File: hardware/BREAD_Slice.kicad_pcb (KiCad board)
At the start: 2 copper layers, 70 x 100 mm, 18 parts, among them J1 Conn_01x10_Female, J2 Screw_Terminal_01x02, J3 Screw_Terminal_01x02, U1 AP63205

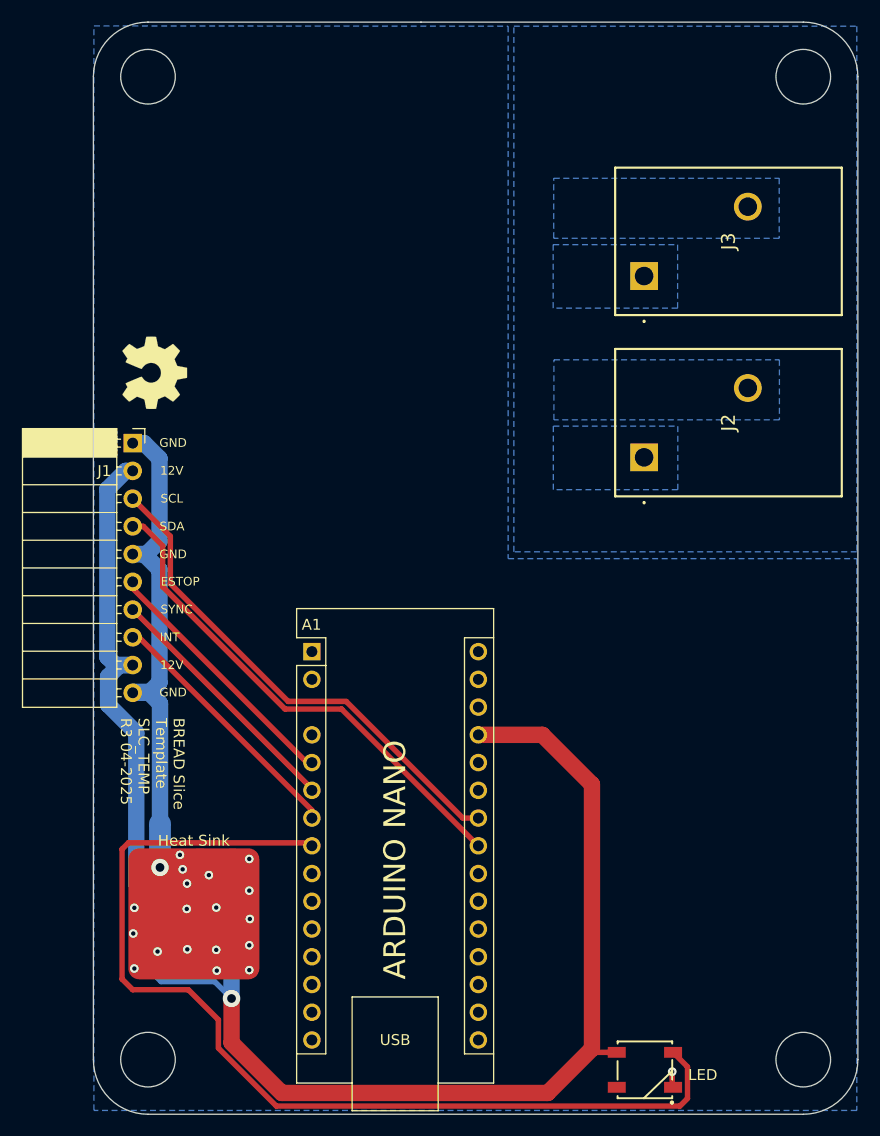
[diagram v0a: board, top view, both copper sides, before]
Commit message: completed board
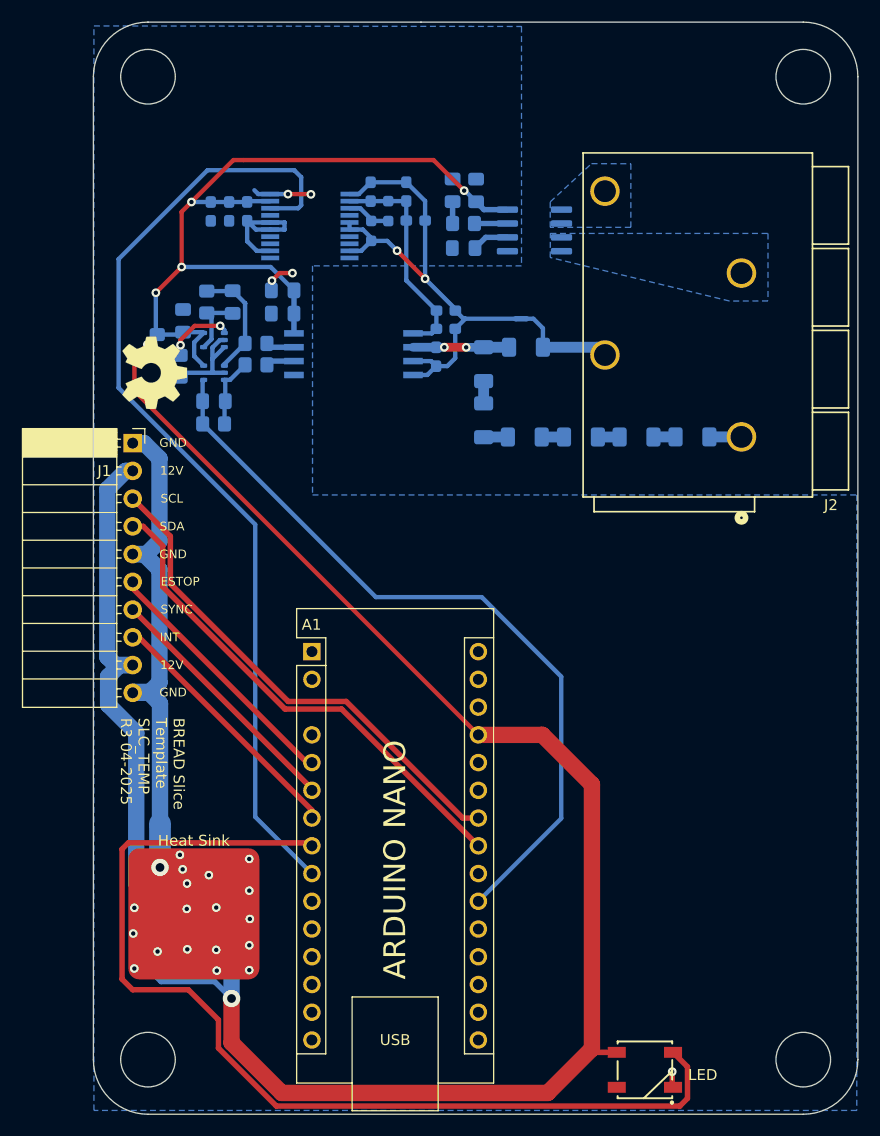
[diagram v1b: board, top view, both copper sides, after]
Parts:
- removed J3: Screw_Terminal_01x02, CRx:Pheonix Conn Term TDPT 4 2-SP-6,35-ZB
- added C10: 100n, Capacitor_SMD:C_0603_1608Metric_Pad1.08x0.95mm_HandSolder, B.Cu at (154.9, 67.9)
- added C11: 0.1u, Capacitor_SMD:C_0603_1608Metric_Pad1.08x0.95mm_HandSolder, B.Cu at (152.1, 58.0)
- added C12: 100p, Capacitor_SMD:C_0603_1608Metric_Pad1.08x0.95mm_HandSolder, B.Cu at (154.0, 70.4)
- added C13: 10n, Capacitor_SMD:C_0603_1608Metric_Pad1.08x0.95mm_HandSolder, B.Cu at (148.0, 55.3)
- added C14: 10n, Capacitor_SMD:C_0603_1608Metric_Pad1.08x0.95mm_HandSolder, B.Cu at (136.7, 57.1)
- added C15: 0.1u, Capacitor_SMD:C_0603_1608Metric_Pad1.08x0.95mm_HandSolder, B.Cu at (135.0, 57.1)
- added C16: 330p, Capacitor_SMD:C_0805_2012Metric_Pad1.18x1.45mm_HandSolder, B.Cu at (135.3, 65.4)
- added C17: 10u, Capacitor_SMD:C_0603_1608Metric_Pad1.08x0.95mm_HandSolder, B.Cu at (133.3, 57.1)
- added C18: 1u, Capacitor_SMD:C_0805_2012Metric_Pad1.18x1.45mm_HandSolder, B.Cu at (139.9, 66.5)
- added C19: 330p, Capacitor_SMD:C_0805_2012Metric_Pad1.18x1.45mm_HandSolder, B.Cu at (133.6, 74.5)
- added C20: 100n, Capacitor_SMD:C_0805_2012Metric_Pad1.18x1.45mm_HandSolder, B.Cu at (139.9, 64.4)
- added C21: 0.1u, Capacitor_SMD:C_0805_2012Metric_Pad1.18x1.45mm_HandSolder, B.Cu at (130.8, 67.2)
- added C5: 1n, Capacitor_SMD:C_0805_2012Metric_Pad1.18x1.45mm_HandSolder, B.Cu at (155.5, 55.2)
- added C6: 0.1u, Capacitor_SMD:C_0805_2012Metric_Pad1.18x1.45mm_HandSolder, B.Cu at (157.6, 55.2)
- added C7: 1n, Capacitor_SMD:C_0805_2012Metric_Pad1.18x1.45mm_HandSolder, B.Cu at (156.5, 60.5)
- added C8: 1u, Capacitor_SMD:C_0603_1608Metric_Pad1.08x0.95mm_HandSolder, B.Cu at (154.9, 66.2)
- added C9: 10u, Capacitor_SMD:C_0603_1608Metric_Pad1.08x0.95mm_HandSolder, B.Cu at (151.2, 55.3)
- added NT2: NetTie_2, NetTie:NetTie-2_SMD_Pad0.5mm, B.Cu at (161.8, 67.0)
- added R1: 1k, Resistor_SMD:R_0805_2012Metric_Pad1.20x1.40mm_HandSolder, B.Cu at (156.5, 58.2)
- added R2: 16.9k, Resistor_SMD:R_0603_1608Metric_Pad0.98x0.95mm_HandSolder, B.Cu at (149.6, 57.1)
- added R3: 10k, Resistor_SMD:R_0603_1608Metric_Pad0.98x0.95mm_HandSolder, B.Cu at (148.0, 58.9)
- added R4: 3.3k, Resistor_SMD:R_0805_2012Metric_Pad1.20x1.40mm_HandSolder, B.Cu at (137.5, 71.2)
- added R5: 3.3k, Resistor_SMD:R_0805_2012Metric_Pad1.20x1.40mm_HandSolder, B.Cu at (137.5, 69.2)
- added R6: 3.3k, Resistor_SMD:R_0805_2012Metric_Pad1.20x1.40mm_HandSolder, B.Cu at (133.0, 65.4)
- added R7: 10k, Resistor_SMD:R_0805_2012Metric_Pad1.20x1.40mm_HandSolder, B.Cu at (128.4, 69.4)
- added R8: 10k, Resistor_SMD:R_0805_2012Metric_Pad1.20x1.40mm_HandSolder, B.Cu at (130.5, 71.3)
- added R9: 3.3k, Resistor_SMD:R_0805_2012Metric_Pad1.20x1.40mm_HandSolder, B.Cu at (133.6, 76.6)
- added RSNS1: 20.05k 1%, Resistor_SMD:R_1206_3216Metric_Pad1.30x1.75mm_HandSolder, B.Cu at (162.2, 69.6)
- added RX1: 665k 1%, Resistor_SMD:R_1206_3216Metric_Pad1.30x1.75mm_HandSolder, B.Cu at (177.5, 77.8)
- added RX2: 665k 1%, Resistor_SMD:R_1206_3216Metric_Pad1.30x1.75mm_HandSolder, B.Cu at (172.3, 77.8)
- added RX3: 665k 1%, Resistor_SMD:R_1206_3216Metric_Pad1.30x1.75mm_HandSolder, B.Cu at (167.2, 77.8)
- added RX4: 665k 1%, Resistor_SMD:R_1206_3216Metric_Pad1.30x1.75mm_HandSolder, B.Cu at (162.1, 77.8)
- added RX5: 665k 1%, Resistor_SMD:R_1206_3216Metric_Pad1.30x1.75mm_HandSolder, B.Cu at (158.3, 76.3)
- added RX6: 665k 1%, Resistor_SMD:R_1206_3216Metric_Pad1.30x1.75mm_HandSolder, B.Cu at (158.3, 71.1)
- added U2: ACS724xLCTR-50AB, Package_SO:SOIC-8_3.9x4.9mm_P1.27mm, B.Cu at (163.0, 58.9)
- added U3: AMC1311BDWVR, kml-custom:DWV0008A, B.Cu at (146.4, 70.2)
- added U4: ADUM5010ARSZ-RL7, kml-custom:RS_20_ADI, B.Cu at (142.4, 58.5)
- added U5: TLV9001IDCK, Package_TO_SOT_SMD:SOT-353_SC-70-5, B.Cu at (133.6, 68.9)
- added U6: TLV9001IDCK, Package_TO_SOT_SMD:SOT-353_SC-70-5, B.Cu at (133.7, 71.9)
- J2: value Screw_Terminal_01x02 -> 2606-1104/010-000; footprint CRx:Pheonix Conn Term TDPT 4 2-SP-6,35-ZB -> kml-custom:CONN4_2606-1104&slash_010-000_WAG
- moved J2 9.11 mm to (181.9, 77.8)
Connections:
- A1 pad 20: /CURR2 -> unconnected-(A1-A1-Pad20)
- A1 pad 21: unconnected-(A1-A2-Pad21) -> /VOLT1
- A1 pad 9: unconnected-(A1-D6-Pad9) -> /ISO_DIS
- J2 pad 1: /Input1+ -> /Isolated DC Voltage Sensor1/DC_BUS+
- J2 pad 2: /Input1- -> /Isolated DC Voltage Sensor1/DC_BUS-
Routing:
- net +5V: track 104.2 -> 231.1 mm, vias 1 -> 6
- net /ISO_DIS: track 0.00 -> 89.5 mm
- net /VOLT1: track 0.00 -> 70.2 mm
- net /Isolated DC Voltage Sensor1/GNDISO: track 0.00 -> 47.9 mm, vias 0 -> 2
- net GND: track 16.8 -> 46.9 mm, vias 20 -> 24
- net /Isolated DC Voltage Sensor1/VDD_ISO: track 0.00 -> 20.4 mm
- net Net-(U6-+): track 0.00 -> 10.5 mm
- net /Isolated DC Voltage Sensor1/DC_BUS-: track 0.00 -> 9.57 mm
- net /Isolated DC Voltage Sensor1/VIN: track 0.00 -> 8.81 mm, vias 0 -> 2
- net Net-(U5-+): track 0.00 -> 8.53 mm, vias 0 -> 2
- net /Isolated DC Voltage Sensor1/VREF: track 0.00 -> 6.63 mm
- net Net-(U6--): track 0.00 -> 6.55 mm
- net /Isolated DC Voltage Sensor1/VSEL: track 0.00 -> 4.13 mm
- net Net-(U2-FILTER): track 0.00 -> 3.38 mm
- net /Isolated DC Voltage Sensor1/DC_BUS+: track 0.00 -> 2.94 mm
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- added copper zone on B.Cu, net /Invasive Isolated AC-DC Current Sensor1/IC_CS_Input+
- added copper zone on B.Cu, net /Invasive Isolated AC-DC Current Sensor1/IC_CS_Input-
- removed copper zone on B.Cu, net (none)
- removed copper zone on B.Cu, net /Input1+
- removed copper zone on B.Cu, net /Input1-
- removed copper zone on B.Cu, net /Input2+
- removed copper zone on B.Cu, net /Input2-
